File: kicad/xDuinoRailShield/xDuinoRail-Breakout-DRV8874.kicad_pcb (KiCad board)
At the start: 2 copper layers, 13.3 x 24.1 mm, 13 parts, among them J101 Conn_01x09, U2901 DRV8874PWPR

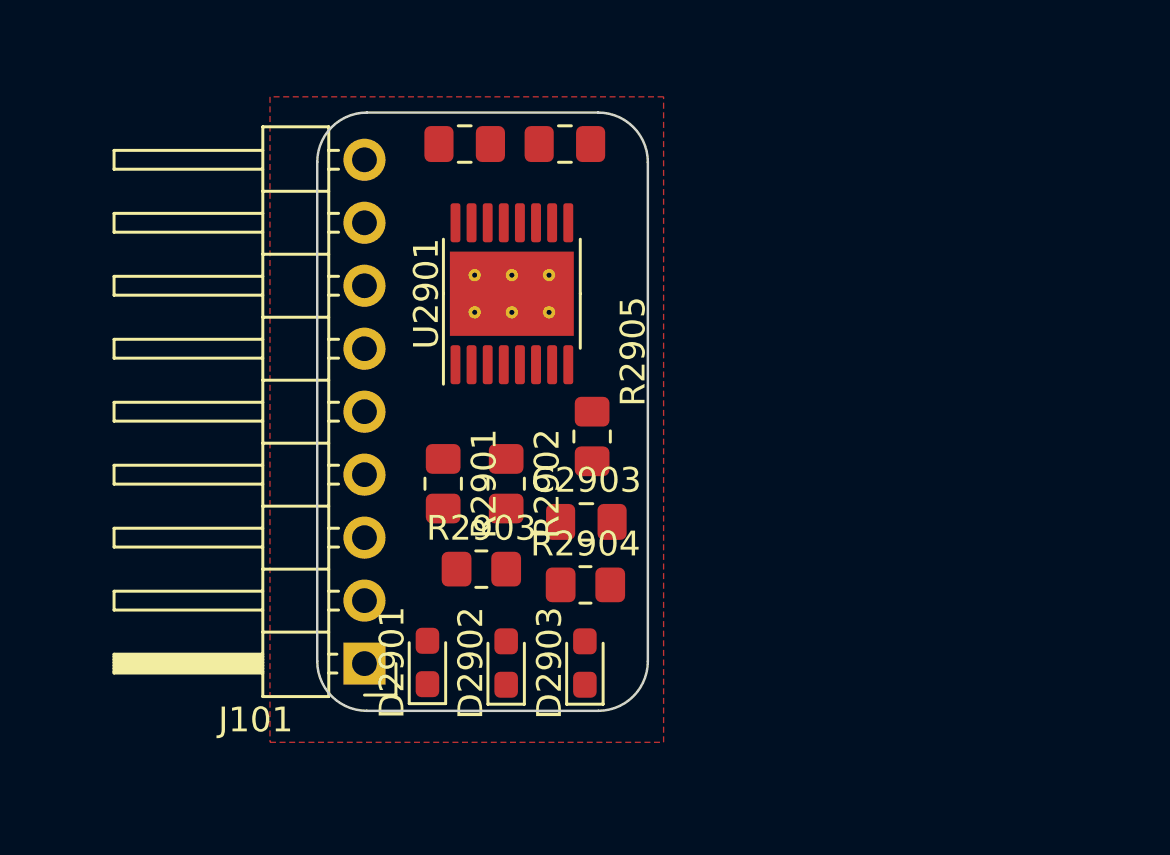
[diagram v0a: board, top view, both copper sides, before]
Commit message: Neue Breakouts
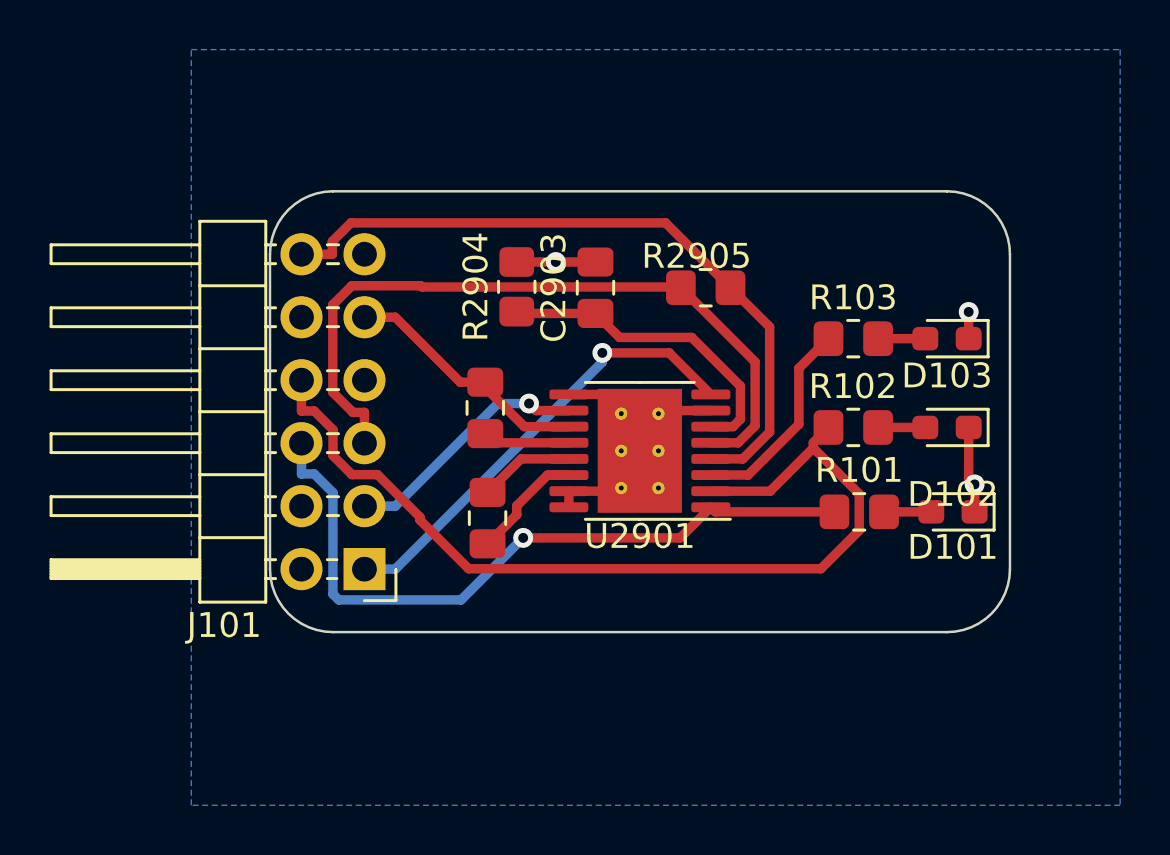
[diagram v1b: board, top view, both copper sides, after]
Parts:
- removed D2901: LED_RED, LED_SMD:LED_0603_1608Metric_Pad1.05x0.95mm_HandSolder
- removed D2902: LED_YELLOW, LED_SMD:LED_0603_1608Metric_Pad1.05x0.95mm_HandSolder
- removed D2903: LED_GREEN, LED_SMD:LED_0603_1608Metric_Pad1.05x0.95mm_HandSolder
- removed R2901, R2902, R2903: 470R, Resistor_SMD:R_0805_2012Metric_Pad1.20x1.40mm_HandSolder
- added D101: LED_RED, LED_SMD:LED_0603_1608Metric_Pad1.05x0.95mm_HandSolder, F.Cu at (160.9, 84.7)
- added D102: LED_YELLOW, LED_SMD:LED_0603_1608Metric_Pad1.05x0.95mm_HandSolder, F.Cu at (160.7, 81.3)
- added D103: LED_GREEN, LED_SMD:LED_0603_1608Metric_Pad1.05x0.95mm_HandSolder, F.Cu at (160.7, 77.7)
- added R101: 470R, Resistor_SMD:R_0805_2012Metric_Pad1.20x1.40mm_HandSolder, F.Cu at (157.1, 84.7)
- added R102: 470R, Resistor_SMD:R_0805_2012Metric_Pad1.20x1.40mm_HandSolder, F.Cu at (156.9, 81.3)
- added R103: 470R, Resistor_SMD:R_0805_2012Metric_Pad1.20x1.40mm_HandSolder, F.Cu at (156.9, 77.7)
- J101: value Conn_01x09 -> Conn_02x06_Odd_Even; footprint Connector_PinHeader_2.54mm:PinHeader_1x09_P2.54mm_Horizontal -> Connector_PinHeader_2.54mm:PinHeader_2x06_P2.54mm_Horizontal
- moved C2902 15.4 mm to (142.1, 84.9), turned to -90 degrees
- moved R2904 12.3 mm to (143.3, 75.6), turned to 90 degrees
- moved C2901 10.7 mm to (142.0, 80.5), turned to 90 degrees
- moved C2903 9.45 mm to (146.5, 75.6), turned to 90 degrees
- moved U2901 8.17 mm to (148.3, 82.2), turned to 180 degrees
- moved R2905 7.55 mm to (150.9, 75.6), turned to 0 degrees
- moved J101 3.81 mm to (137.2, 87.0)
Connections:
- J101 pad 1: /centrale-driver-8874/BRAKE -> /DCC0
- J101 pad 2: /centrale-driver-8874/DIR -> unconnected-(J101-Pin_2-Pad2)
- J101 pad 3: /centrale-driver-8874/PWM -> /DCC1
- J101 pad 4: /centrale-driver-8874/SENSE -> unconnected-(J101-Pin_4-Pad4)
- J101 pad 5: /DCC0 -> +3V3
- J101 pad 6: /DCC1 -> /BRAKE
- J101 pad 7: +VIN -> GND
- J101 pad 8: GND -> /DIR
- J101 pad 9: +3V3 -> +VIN
- U2901 pad 1: /centrale-driver-8874/BRAKE -> /BRAKE
- U2901 pad 2: /centrale-driver-8874/DIR -> /DIR
- U2901 pad 3: /centrale-driver-8874/PWM -> /PWM
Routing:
- net /DIR: track 0.00 -> 37.7 mm
- net +3V3: track 0.00 -> 29.7 mm
- net /BRAKE: track 0.00 -> 28.9 mm, vias 0 -> 1
- net /centrale-driver-8874/SENSE: track 0.00 -> 28.5 mm
- net /DCC0: track 0.00 -> 18.5 mm, vias 0 -> 1
- net GND: track 0.00 -> 15.9 mm, vias 0 -> 3
- net /centrale-driver-8874/iPROP: track 0.00 -> 12.9 mm
- net +VIN: track 0.00 -> 10.2 mm
- net /DCC1: track 0.00 -> 10.1 mm, vias 0 -> 1
- net /PWM: track 0.00 -> 8.35 mm
- net /centrale-driver-8874/CPL: track 0.00 -> 4.64 mm
- net /centrale-driver-8874/CPH: track 0.00 -> 3.84 mm
- net /centrale-driver-8874/VCP: track 0.00 -> 3.53 mm
- net Net-(D103-A): track 0.00 -> 1.91 mm
- net Net-(D102-A): track 0.00 -> 1.91 mm
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- added copper zone on B.Cu, net GND
- removed copper zone on F.Cu, net GND
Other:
- board size 13.3 x 24.1 mm -> 29.8 x 17.8 mm

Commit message: Many exiting news
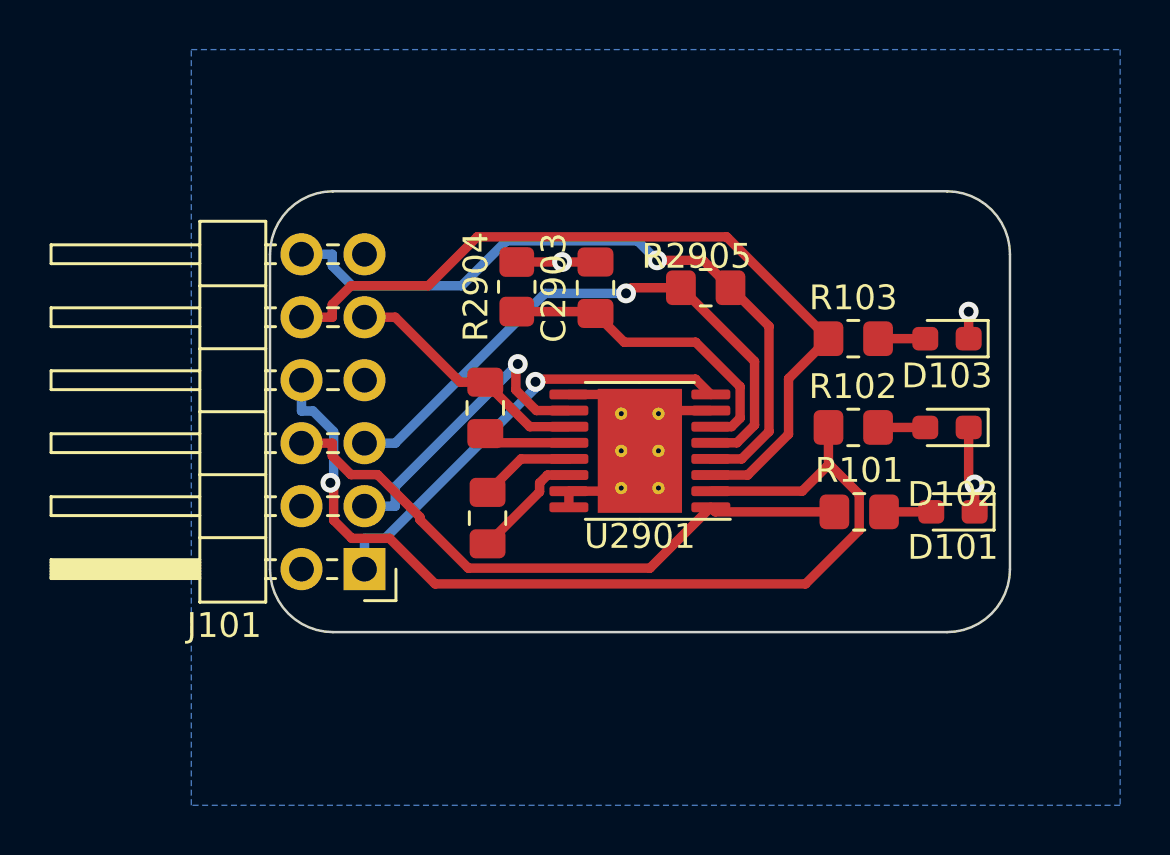
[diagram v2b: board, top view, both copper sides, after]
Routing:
- net /PWM: track 8.35 -> 32.9 mm
- net +3V3: track 29.7 -> 24.2 mm, vias 0 -> 1
- net /BRAKE: track 28.9 -> 25.0 mm, vias 1 -> 0
- net /DCC1: track 10.1 -> 12.6 mm
- net /DIR: track 37.7 -> 39.6 mm, vias 0 -> 1
- net /centrale-driver-8874/SENSE: track 28.5 -> 28.9 mm, vias 0 -> 1
